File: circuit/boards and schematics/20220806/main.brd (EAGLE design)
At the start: 70 x 30 mm, 11 parts, among them U1 ESP32-DEVKITC-32D, X1 JST-XH-05-PIN-LONG-PAD

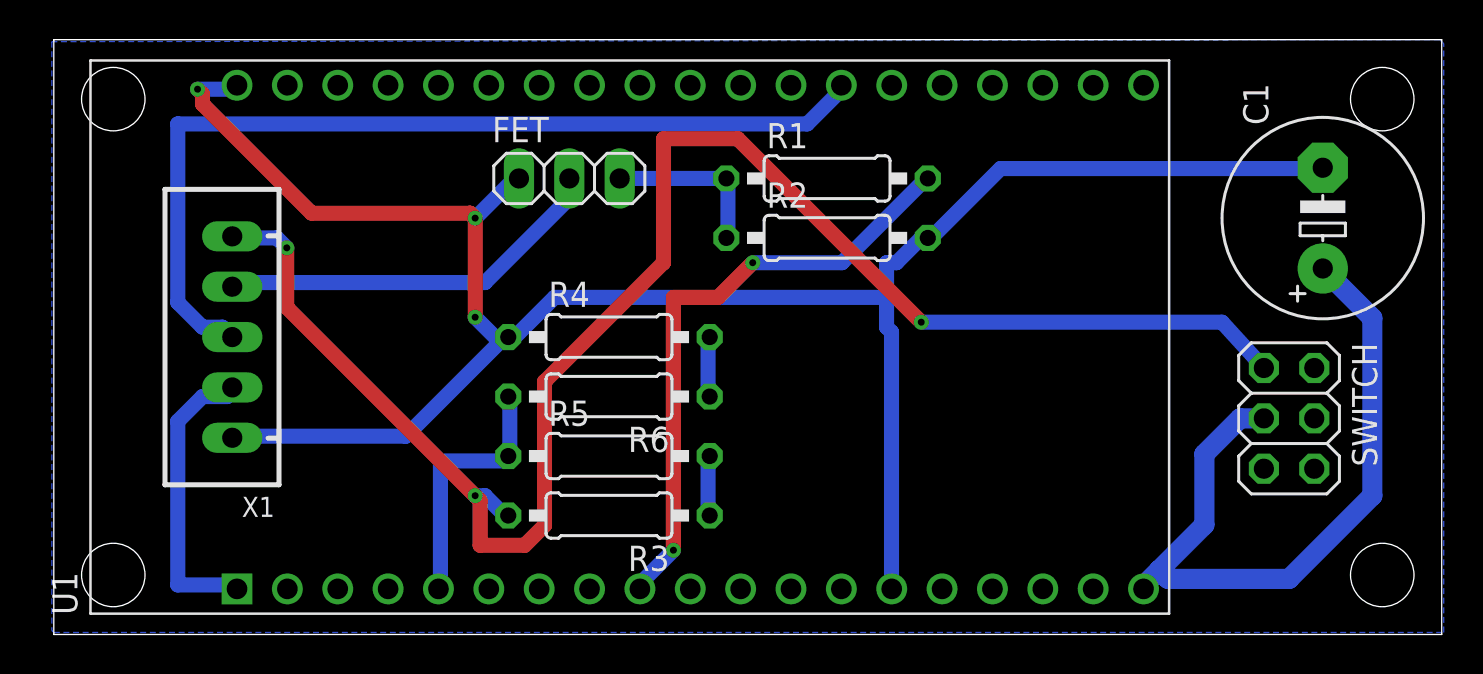
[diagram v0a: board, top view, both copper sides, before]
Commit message: fix some lines
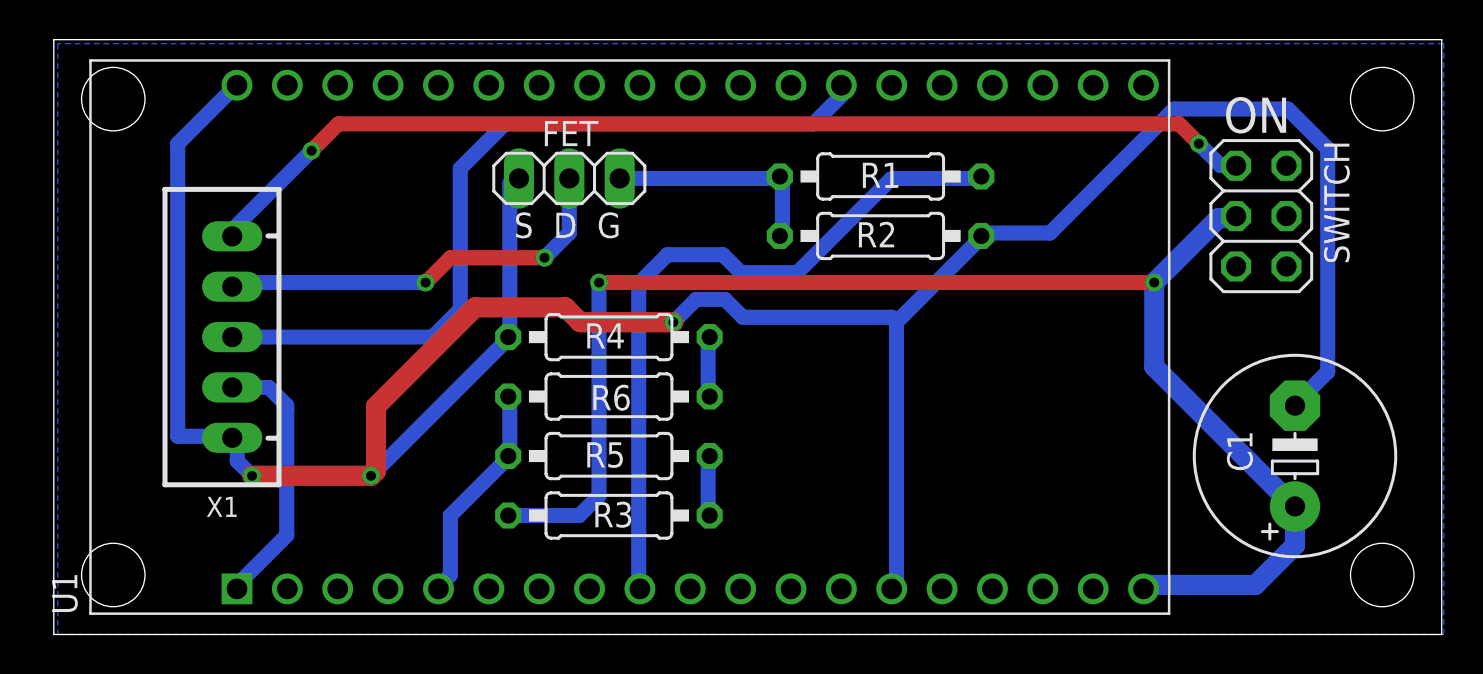
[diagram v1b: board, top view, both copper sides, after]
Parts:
- moved C1 12.1 mm to (62.6, 9.00)
- moved SWITCH 10.3 mm to (60.9, 21.1)
- moved R1 2.70 mm to (41.7, 23.1)
- moved R2 2.70 mm to (41.7, 20.1)
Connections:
- net N$4 renamed HALL_SIGNAL
- net N$6 renamed MOTOR_MINUS
- net N$7 renamed V_CHECK
- removed net N$1: R3.2, SWITCH.1, X1.5
- new net MOTOR_PLUS: SWITCH.1, X1.5
- net +5V: now also R3.2
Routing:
- net N$1: track 84.9 -> 0.00 mm, vias 3 -> 0
- net MOTOR_PLUS: track 0.00 -> 54.2 mm, vias 0 -> 2
- net +5V: track 36.8 -> 74.3 mm, vias 0 -> 2
- net GND: track 105.4 -> 135.8 mm
- net HALL_SIGNAL: track 46.9 -> 40.5 mm
- net N$3: track 30.7 -> 35.8 mm, vias 2 -> 0
- net N$2: track 8.54 -> 11.2 mm
- net V_CHECK: track 13.2 -> 11.3 mm
- net +3V3: track 14.9 -> 13.4 mm
- net MOTOR_MINUS: track 20.0 -> 21.0 mm, vias 0 -> 2
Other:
- board text added: "ON"
- board text added: "S D G"
